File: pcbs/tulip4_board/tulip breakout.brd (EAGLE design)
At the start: 86.3 x 47.6 mm, 51 parts, among them IC1 CP2102N-A02-GQFN24, IC2 LM2937, U1 ESP32-S3-WROOM-2-N32R8V, U2 6N138SDM, U4 UDA1334ATS, X2 FH12-40S-0.5SH, X3 19269, X5 19269, X6 19269

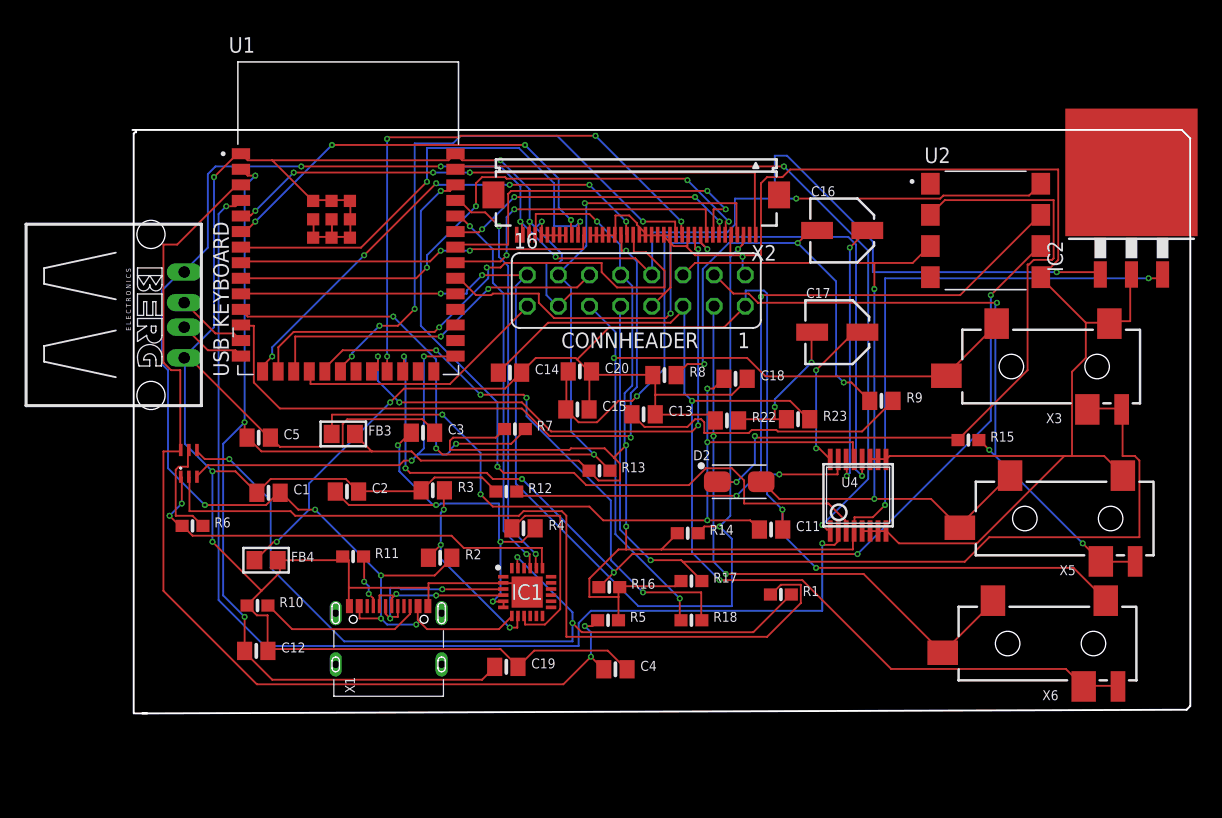
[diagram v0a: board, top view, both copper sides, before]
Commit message: .
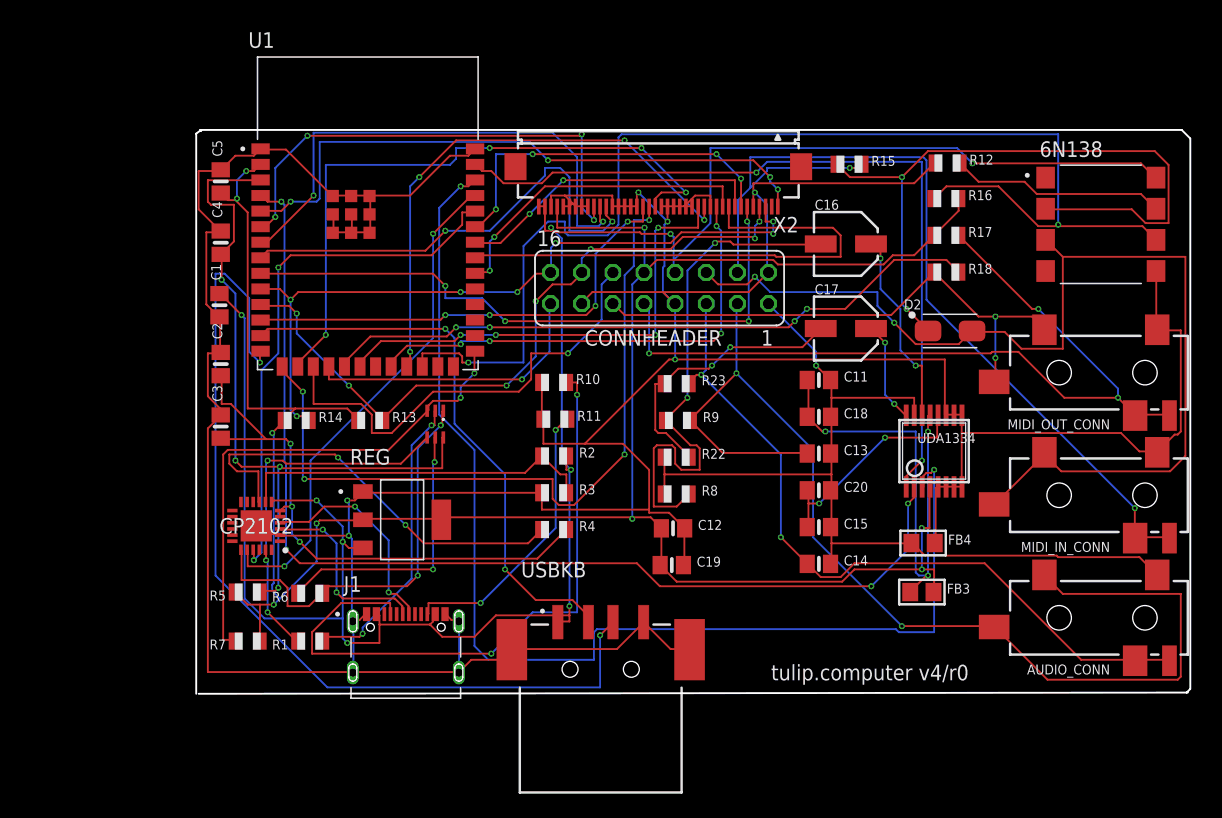
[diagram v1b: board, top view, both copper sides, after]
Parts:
- removed IC1: CP2102N-A02-GQFN24, CP2102N-A02-GQFN24:QFN50P400X400X80-25N
- removed IC2: LM2937, linear:TO263-3
- removed U$6: MBT3904DW1T1G, MBT3904DW1T1G:SOT236
- removed U2: 6N138SDM, 6N138SDM:COUPL_6N138SDM
- removed U4: UDA1334ATS, microbuilder:SSOP16_4.4MM
- removed USB_KEYBOARD: (no value), con-berg:PN87520
- removed X1: (no value), microbuilder:USB_C_CUSB31-CFM2AX-01-X
- removed X3, X5, X6: 19269, microbuilder:4UCONN_19269
- added 6N138: 6N138SDM, 6N138SDM:COUPL_6N138SDM
- added AUDIO_CONN, MIDI_IN_CONN, MIDI_OUT_CONN: 19269, microbuilder:4UCONN_19269
- added CP2102: CP2102N-A02-GQFN24, CP2102N-A02-GQFN24:QFN50P400X400X80-25N
- added J1: CSP-USC16-TR, CSP-USC16-TR:VALCON_CSP-USC16-TR
- added REG: TS1117BCW33_RPG, TS1117BCW33_RPG:VREG_TS1117BCW33_RPG
- added RESET: MBT3904DW1T1G, MBT3904DW1T1G:SOT236
- added UDA1334: UDA1334ATS, microbuilder:SSOP16_4.4MM
- added USBKB: USB-A-S-X-X-SM2, USB-A-S-X-X-SM2:SAMTEC_USB-A-S-X-X-SM2
- R1, R10, R11, R12, R13, R14, R15, R16, R17, R18, R5, R6, R7: device microbuilder:0603-NO -> adafruit:R0805
- R2, R22, R23, R3, R4, R8, R9: device microbuilder:0805-NO -> adafruit:R0805
- moved FB4 53.6 mm to (73.1, 12.9)
- moved FB3 48.9 mm to (73.0, 8.90)
- moved C4 47.4 mm to (15.8, 37.4), turned to 90 degrees
- moved R12 44.9 mm to (75.1, 43.9)
- moved R16 42.0 mm to (75.0, 41.0)
- moved R1 38.6 mm to (23.1, 4.90), turned to 180 degrees
- moved C12 35.4 mm to (52.7, 14.1)
- moved R18 35.2 mm to (75.0, 35.0)
- moved R17 35.0 mm to (75.0, 38.0)
- moved R14 33.2 mm to (22.0, 22.9)
- moved R10 30.3 mm to (43.0, 26.0)
- moved C14 29.6 mm to (64.6, 11.2)
- moved R5 29.5 mm to (18.0, 8.90), turned to 180 degrees
- moved R7 27.8 mm to (18.0, 4.90), turned to 180 degrees
- moved R15 24.5 mm to (67.1, 43.8)
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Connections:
- removed net CC1: R11.2, X1.A5
- removed net CC2: R10.2, X1.B5
- new net N$3: J1.B5, R11.2
- new net N$4: J1.A5, R10.2
- net !DTR: now also CP2102.23, RESET.4; no longer IC1.23, U$6.4
- net !RTS: now also CP2102.19, RESET.1; no longer IC1.19, U$6.1
- net 3V3: now also REG.2, REG.4, UDA1334.4; no longer IC2.3, U4.4
- net 3V3_USB: now also CP2102.5, CP2102.6; no longer IC1.5, IC1.6
- net 5V_USB: now also 6N138.8, CP2102.7, J1.A4, J1.A9, J1.B4, J1.B9, REG.3, USBKB.01; no longer IC1.7, IC2.1, U2.8, USB_KEYBOARD.1, X1.A4B9, X1.B4A9
- net AGND: now also AUDIO_CONN.1, UDA1334.15; no longer U4.15, X6.1
- net BCLK: now also UDA1334.1; no longer U4.1
- net D+: now also USBKB.03; no longer USB_KEYBOARD.3
- net D-: now also USBKB.02; no longer USB_KEYBOARD.2
- net DIN: now also UDA1334.3; no longer U4.3
- net ESP32_EN: now also RESET.6; no longer U$6.6
- net GND: now also 6N138.5, CP2102.2, CP2102.25, J1.A1, J1.A12, J1.B1, J1.B12, J1.S1, J1.S2, J1.S3, J1.S4, MIDI_IN_CONN.1, MIDI_OUT_CONN.1, REG.1, UDA1334.10, UDA1334.11, UDA1334.5, UDA1334.6, UDA1334.7, UDA1334.8, UDA1334.9, USBKB.04, USBKB.S1, USBKB.S2; no longer IC1.2, IC1.25, IC2.2, U2.5, U4.10, U4.11, U4.5, U4.6, U4.7, U4.8, U4.9, USB_KEYBOARD.4, X1.A1B12, X1.B1A12, X3.1, X5.1
- net IO0: now also RESET.3; no longer U$6.3
- net LOUT: now also AUDIO_CONN.2, AUDIO_CONN.4; no longer X6.2, X6.4
- net LRC: now also UDA1334.2; no longer U4.2
- net MIDI_IN: now also 6N138.6; no longer U2.6
- net MIDI_IN_SINK: now also 6N138.3, MIDI_IN_CONN.2, MIDI_IN_CONN.4; no longer U2.3, X5.2, X5.4
- net MIDI_IN_SOURCE: now also MIDI_IN_CONN.3, MIDI_IN_CONN.5; no longer X5.3, X5.5
- net MIDI_OUT_SINK: now also MIDI_OUT_CONN.2, MIDI_OUT_CONN.4; no longer X3.2, X3.4
- net MIDI_OUT_SOURCE: now also MIDI_OUT_CONN.3, MIDI_OUT_CONN.5; no longer X3.3, X3.5
- net N$1: now also RESET.2; no longer U$6.2
- net N$10: now also UDA1334.12; no longer U4.12
- net N$11: now also UDA1334.16; no longer U4.16
- net N$12: now also UDA1334.14; no longer U4.14
- net N$2: now also RESET.5; no longer U$6.5
- net N$30: now also 6N138.2; no longer U2.2
- net N$32: now also 6N138.7; no longer U2.7
- net N$5: now also UDA1334.13; no longer U4.13
- net ROUT: now also AUDIO_CONN.3, AUDIO_CONN.5; no longer X6.3, X6.5
- net UART0_RXD: now also CP2102.21; no longer IC1.21
- net UART0_TXD: now also CP2102.20; no longer IC1.20
- net USBC_D+: now also CP2102.3, J1.A6; no longer IC1.3, X1.A6, X1.B6
- net USBC_D-: now also CP2102.4, J1.A7; no longer IC1.4, X1.A7, X1.B7
- net USB_RESET: now also CP2102.9; no longer IC1.9
- net USB_VBUS: now also CP2102.8; no longer IC1.8
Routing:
- net D+: track 5.61 -> 75.7 mm, vias 0 -> 2
- net AGND: track 137.1 -> 76.1 mm, vias 5 -> 1
- net N$4: track 0.00 -> 52.7 mm, vias 0 -> 2
- net 3V3: track 240.4 -> 190.3 mm, vias 8 -> 9
- net N$1: track 68.5 -> 24.3 mm, vias 0 -> 2
- net N$32: track 60.8 -> 17.5 mm, vias 2 -> 0
- net N$10: track 60.6 -> 17.7 mm
- net D-: track 5.91 -> 45.8 mm, vias 0 -> 2
- net !DTR: track 69.5 -> 30.8 mm
- net SCL: track 96.9 -> 59.5 mm, vias 4 -> 7
- net DIN: track 60.5 -> 96.5 mm
- net N$5: track 68.1 -> 40.3 mm, vias 5 -> 3
- net ROUT: track 87.5 -> 60.2 mm
- net MIDI_IN_SINK: track 64.1 -> 88.1 mm
- net N$3: track 0.00 -> 23.2 mm, vias 0 -> 2
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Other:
- board size 86.3 x 47.6 mm -> 81.1 x 46 mm
- board text added: "tulip.computer v4/r0"
